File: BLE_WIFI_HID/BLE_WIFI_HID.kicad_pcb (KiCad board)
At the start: 2 copper layers, 62.9 x 33.4 mm, 25 parts, among them J1 Conn_02x03_Odd_Even, J2 Conn_02x03_Odd_Even, P3 PROGRAMMER SERIAL, P4 Battery, U1 ESP32-WROOM, U2 AP2112K-3.3TRG1, U3 MCP73831T-2ACI/OT

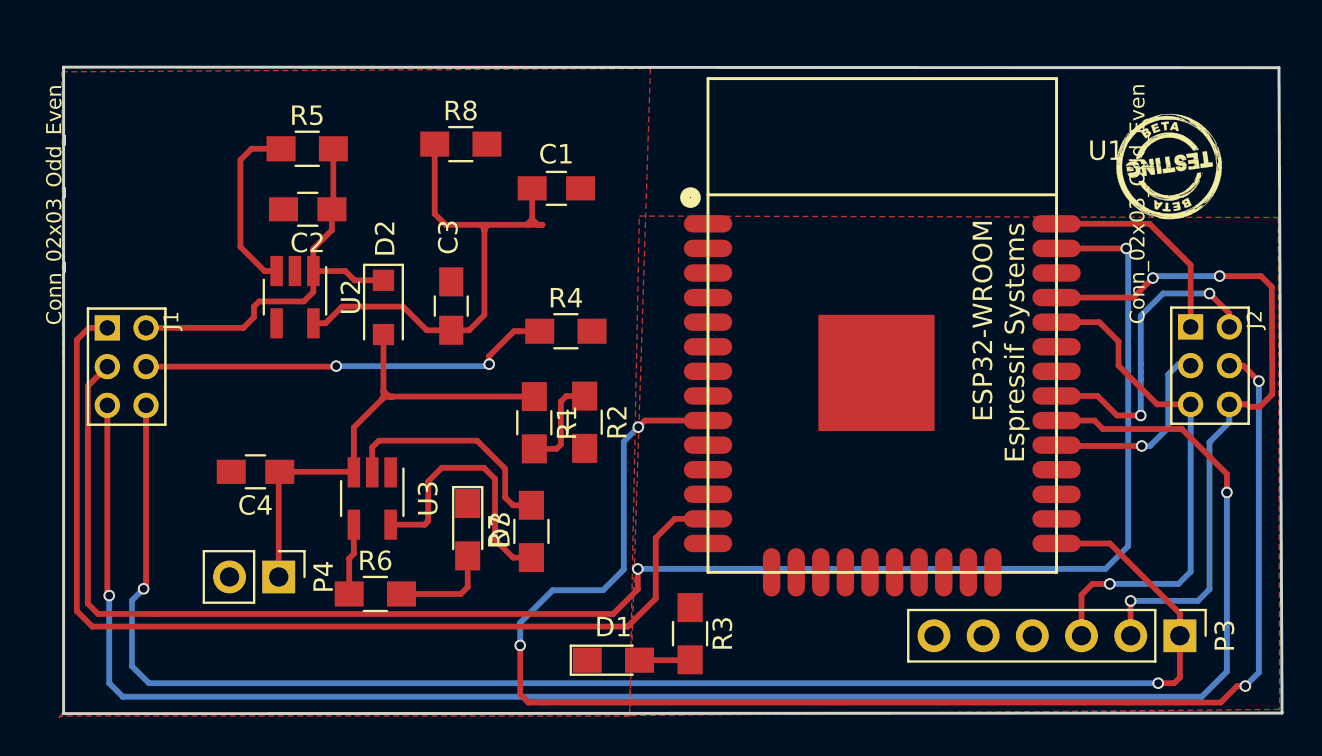
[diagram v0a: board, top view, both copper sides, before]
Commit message: re-routeo
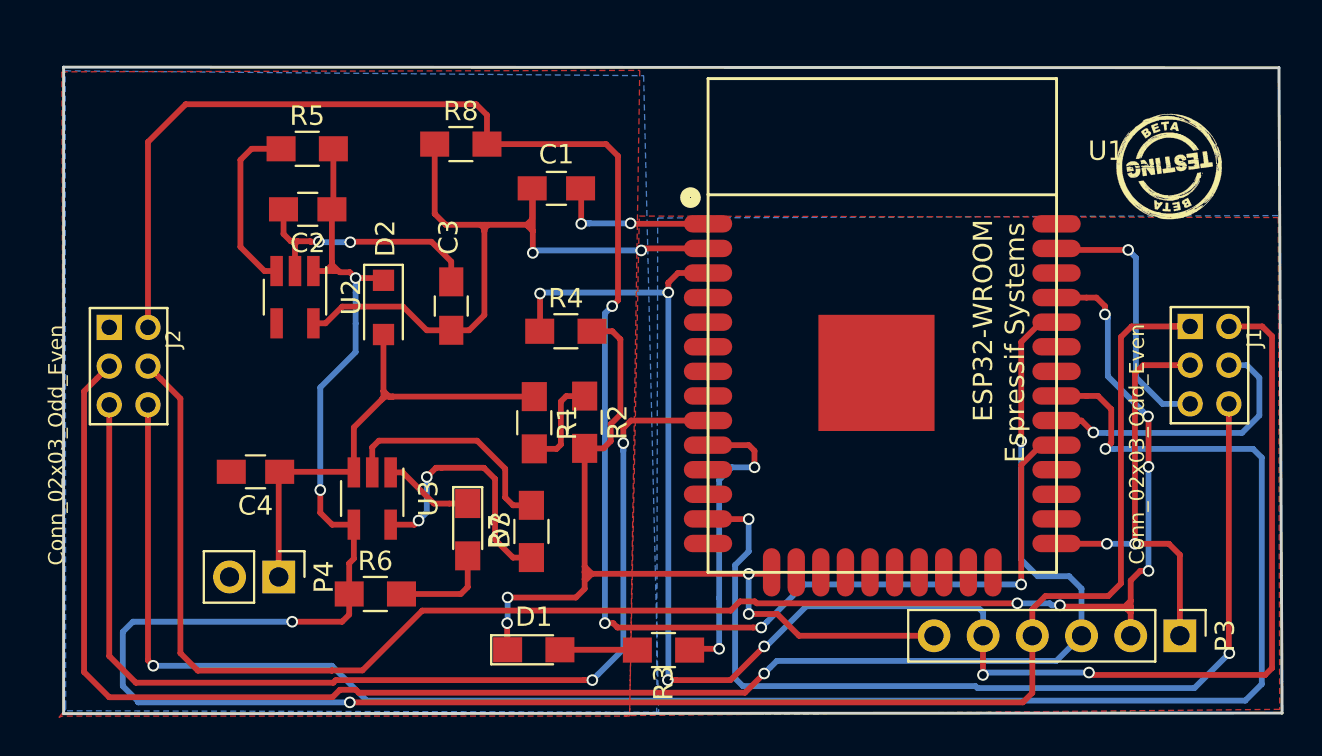
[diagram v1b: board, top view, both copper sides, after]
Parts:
- moved J1 55.9 mm to (204.9, 92.7)
- moved J2 55.9 mm to (149.1, 92.8)
- moved D1 4.15 mm to (170.0, 107.4)
- moved R3 1.61 mm to (176.7, 107.4), turned to 180 degrees
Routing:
- net VCC: track 25.1 -> 120.4 mm, vias 0 -> 4
- net /ESP_CS: track 10.4 -> 92.0 mm, vias 1 -> 4
- net /ESP_RTS: track 16.1 -> 97.2 mm
- net /SCK: track 93.1 -> 14.9 mm, vias 2 -> 1
- net /MISO: track 87.7 -> 13.8 mm, vias 2 -> 1
- net /ESP_RESET: track 21.3 -> 87.4 mm, vias 2 -> 6
- net /ESP_RX: track 26.3 -> 89.5 mm, vias 1 -> 2
- net /ESP_GPIO0: track 79.6 -> 22.6 mm
- net GND: track 11.0 -> 67.7 mm, vias 0 -> 8
- net /ESP_TX: track 36.0 -> 88.6 mm, vias 3 -> 6
- net /ESP_BUSY: track 77.5 -> 57.2 mm, vias 4 -> 2
- net /IO25: track 0.00 -> 15.7 mm, vias 0 -> 2
- net +3V3: track 27.4 -> 38.9 mm, vias 0 -> 2
- net Net-(D3-Pad1): track 0.00 -> 4.65 mm
- net /MOSI: track 52.9 -> 50.0 mm, vias 0 -> 2
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- added copper zone on B.Cu, net GND
